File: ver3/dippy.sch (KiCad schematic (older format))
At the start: 28 parts, among them J1 Conn_01x02_Female, J2 Screw_Terminal_01x03, J3 Screw_Terminal_01x04, J4 Conn_Coaxial, J5 Conn_02x03_Odd_Even, J6 Screw_Terminal_01x04, J7 Conn_01x02_Female, U1 ATmega328P-PU-C, U2 RFM95W-915S2, U3 MCP1700-3302E_SOT23, Y1 Crystal

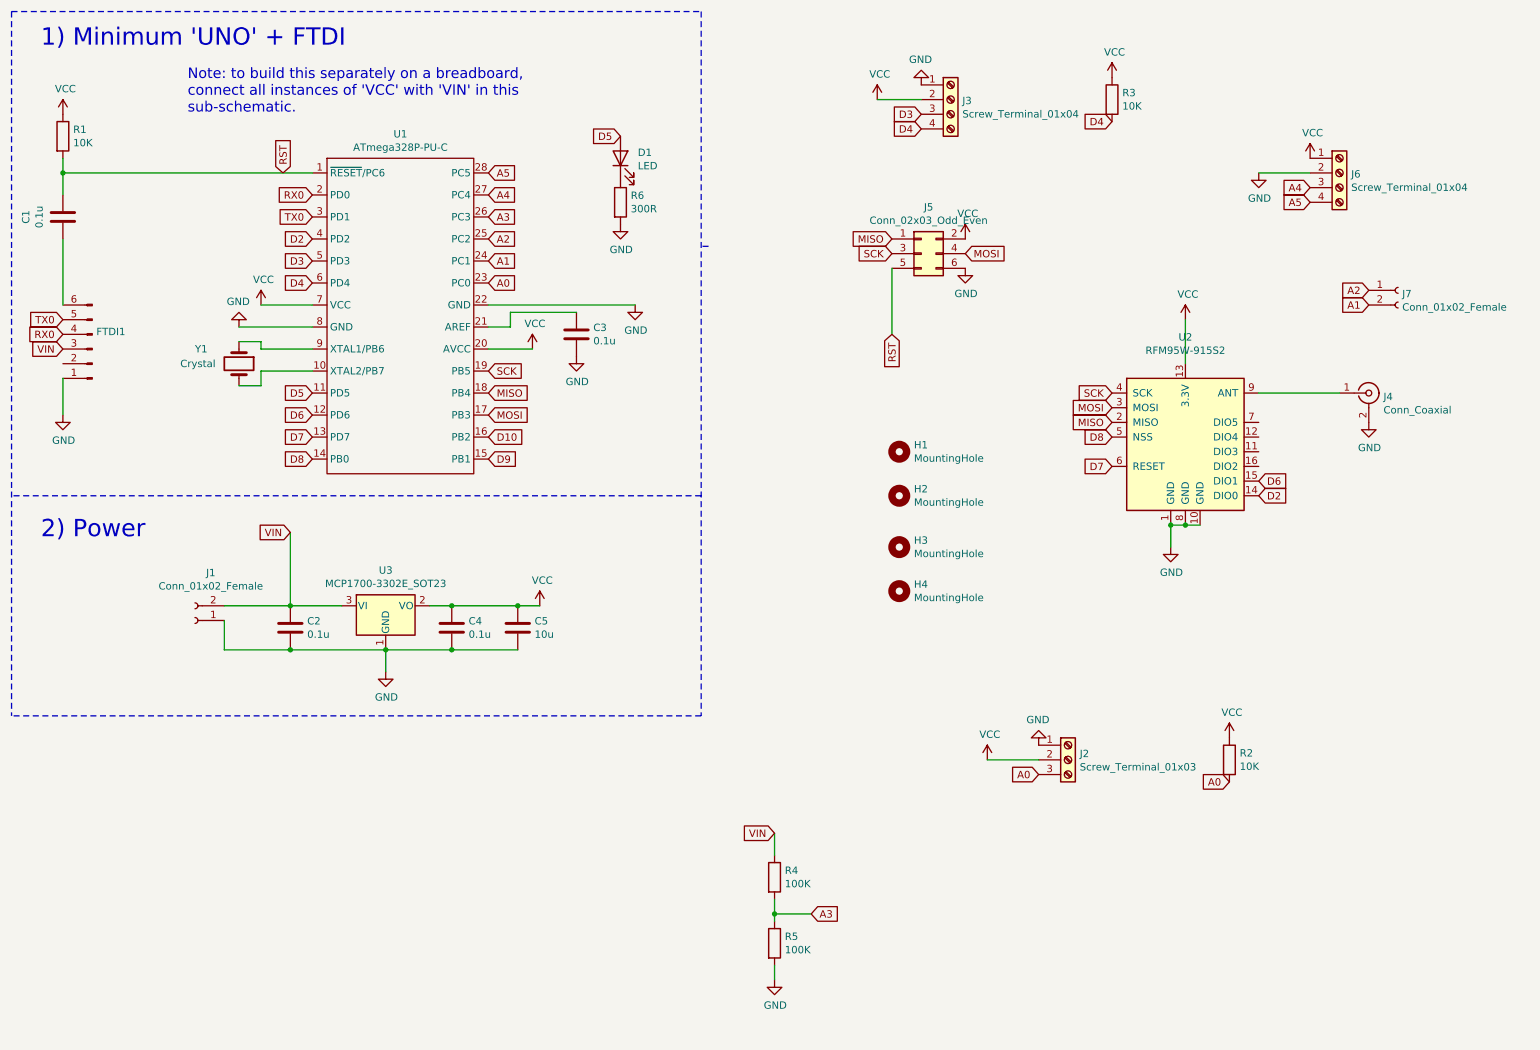
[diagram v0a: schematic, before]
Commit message: update
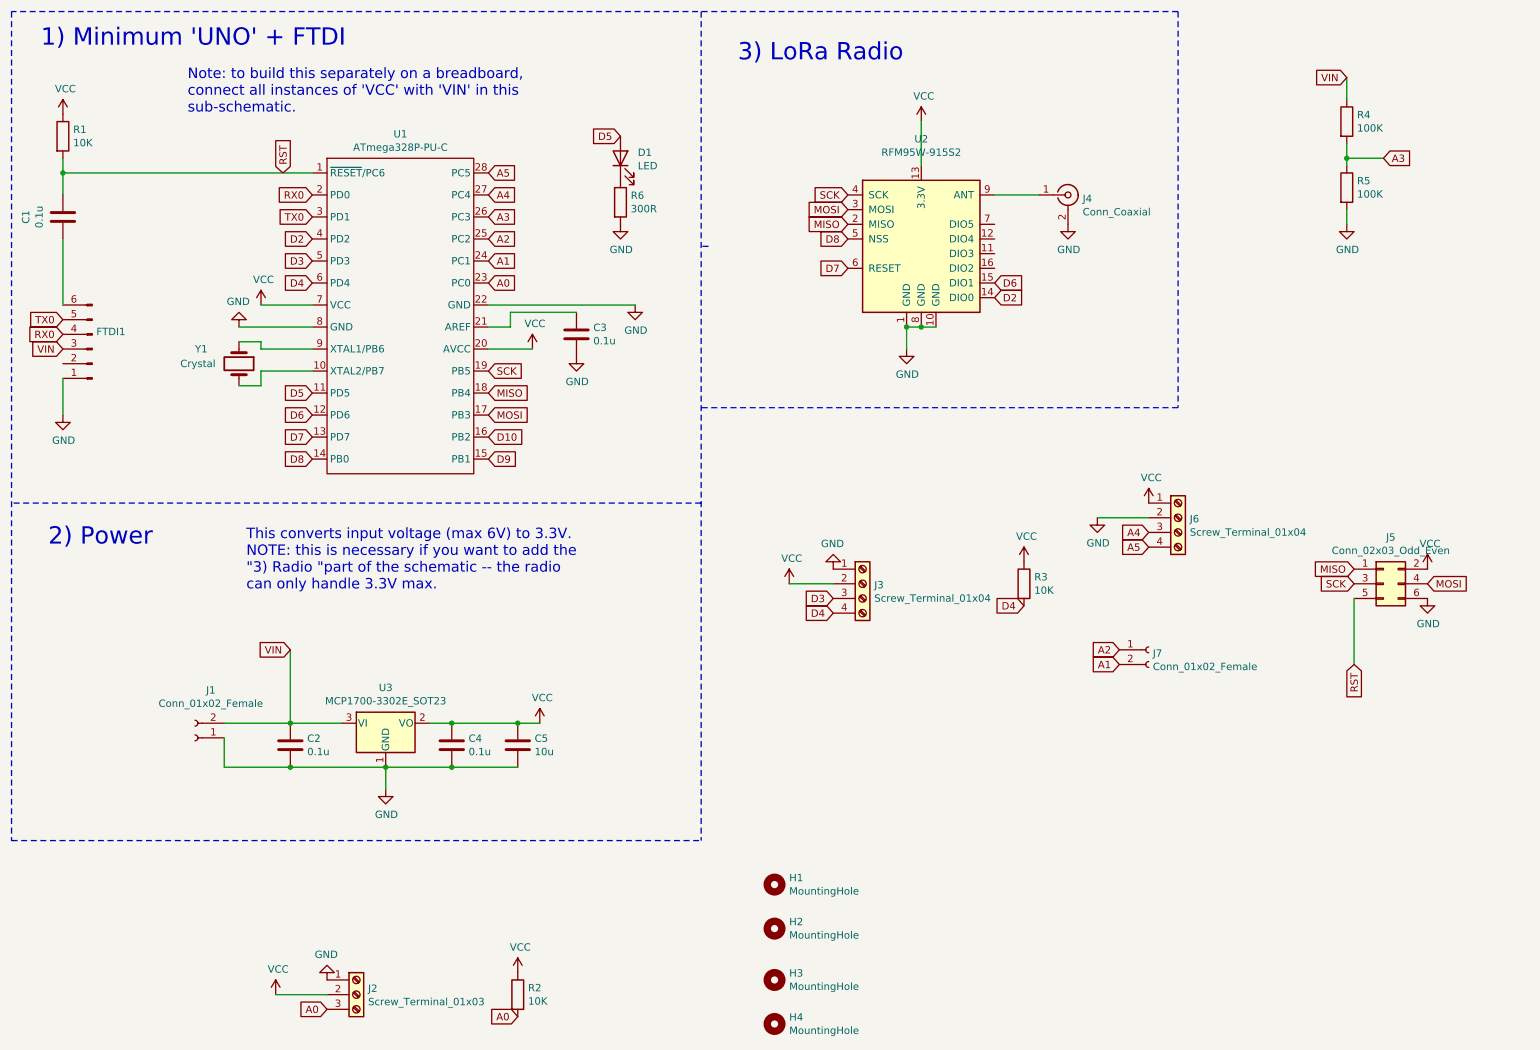
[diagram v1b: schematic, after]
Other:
- note added: "3) LoRa Radio"
- note added: "This converts input voltage (max 6V) to 3.3V. \nNOTE: this is necessary if you want to add the \n"3) Radio "part of the schematic -- the radio \ncan only handle 3.3V max."
- moved on the sheet: C2, C4, C5, H1, H2, H3, H4, J1, J2, J3, J4, J5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

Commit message: update
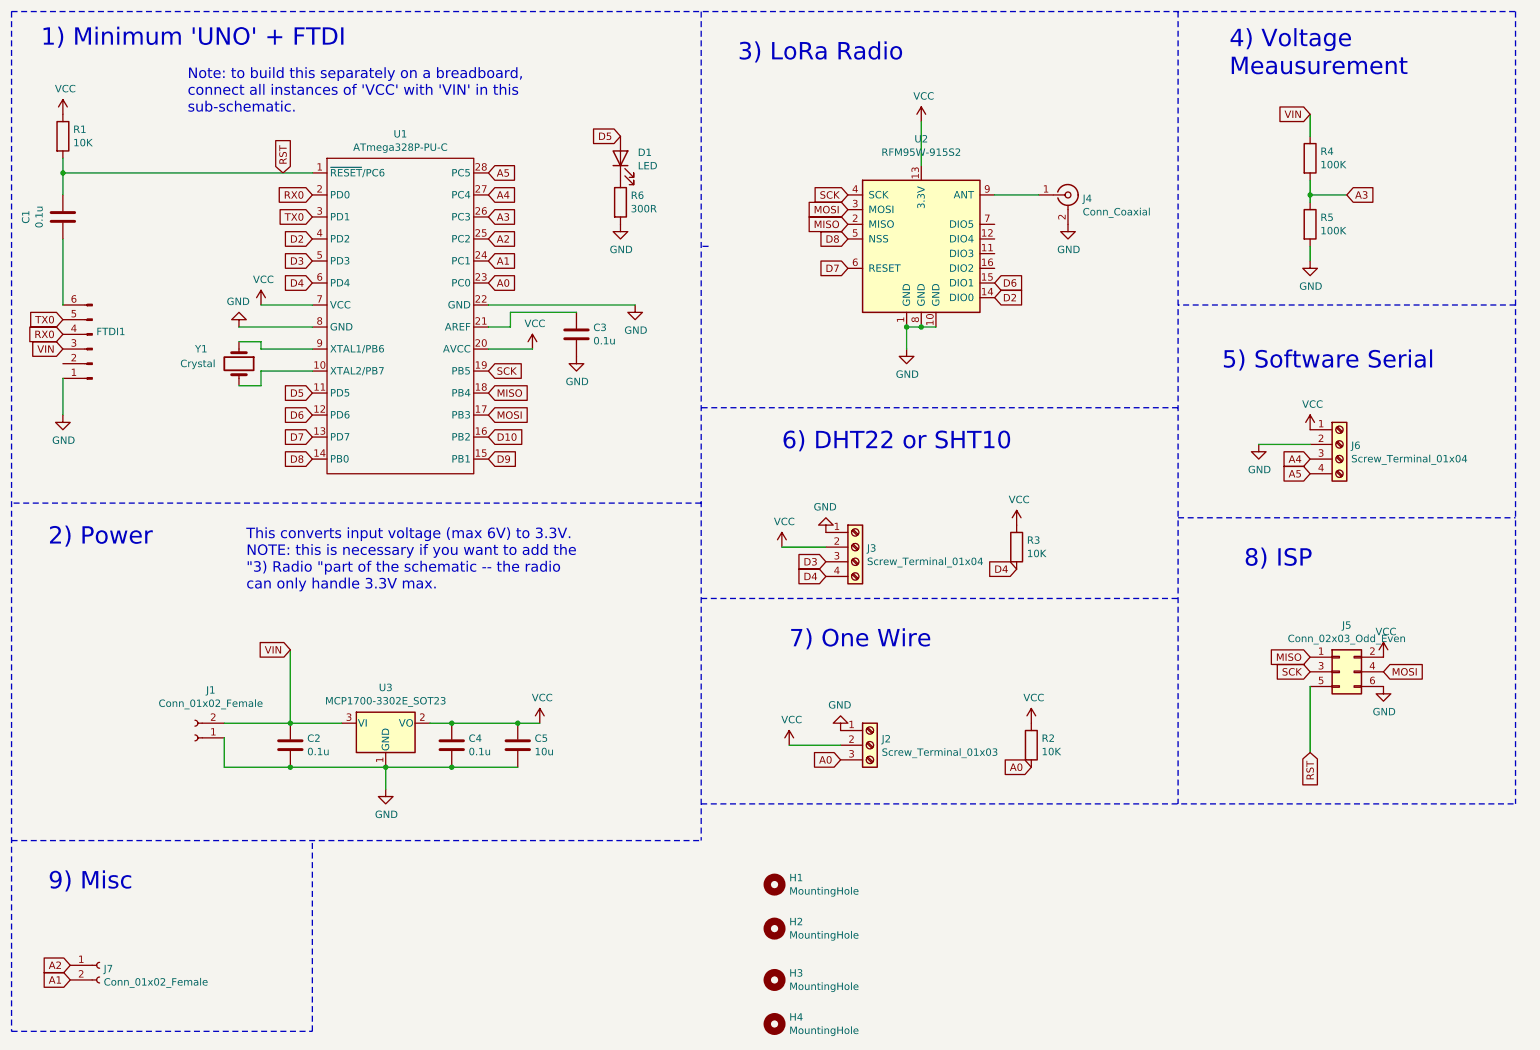
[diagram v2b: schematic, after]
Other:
- note added: "4) Voltage\nMeausurement"
- note added: "5) Software Serial"
- note added: "6) DHT22 or SHT10"
- note added: "7) One Wire"
- note added: "8) ISP"
- note added: "9) Misc"
- moved on the sheet: J2, J3, J5, J6, J7, R2, R3, R4, R5
